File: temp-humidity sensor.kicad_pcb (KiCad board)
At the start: 2 copper layers, 36 parts, among them J1 Conn_01x02, J2 USB_C_Receptacle_USB2.0_16P, SW1 SW_Push, SW2 SW_Push, SW3 SS-12D01-G040, U1 SHT4x, U2 ESP32-C6-WROOM-1, U3 BQ24074RGT, U4 USBLC6-2SC6, U5 TPS63031DSK

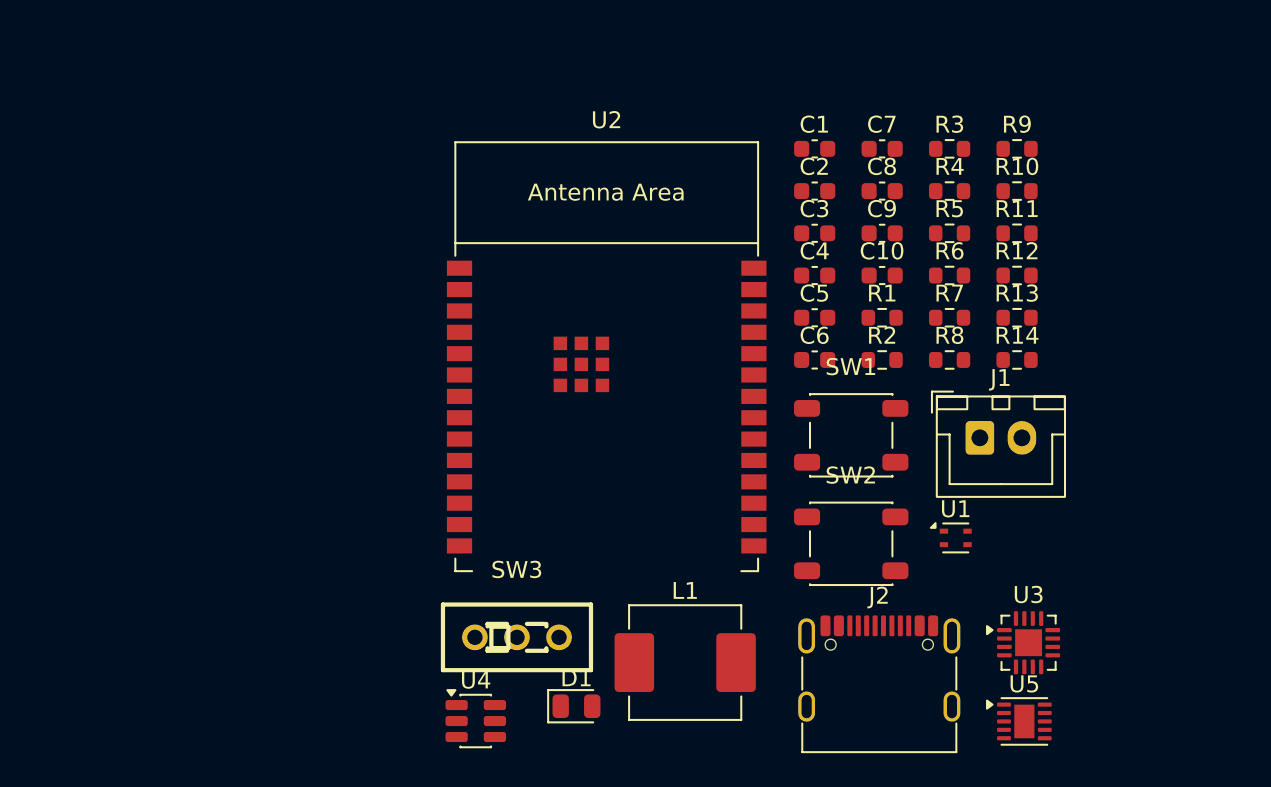
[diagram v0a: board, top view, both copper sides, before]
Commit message: Working On PCB
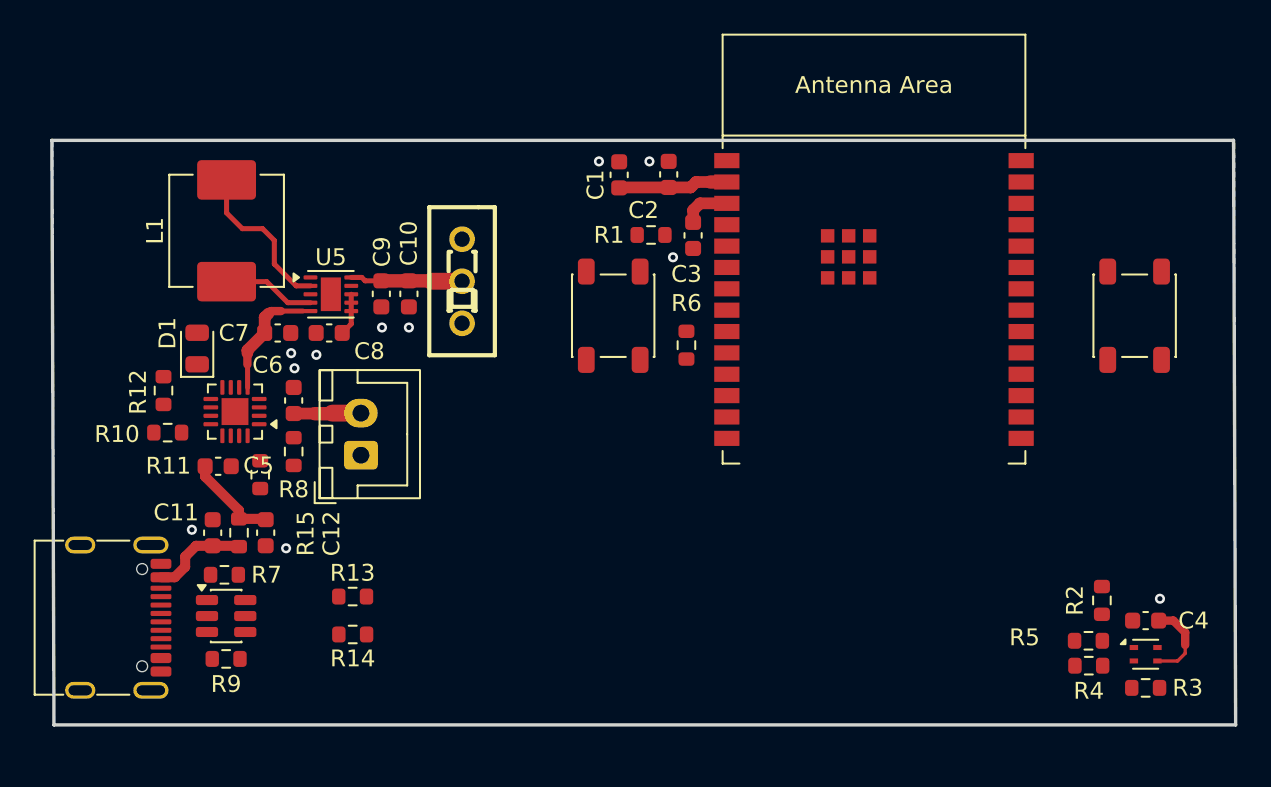
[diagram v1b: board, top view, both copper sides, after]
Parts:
- added C11: 470n, Capacitor_SMD:C_0603_1608Metric, F.Cu at (105.4, 94.6)
- added C12: 470n, Capacitor_SMD:C_0603_1608Metric, F.Cu at (108.6, 94.6)
- added R15: 0R, Resistor_SMD:R_0603_1608Metric, F.Cu at (107.0, 94.6)
- C10: value 10u -> 100n
- moved R9 56.0 mm to (106.2, 102.1), turned to 180 degrees
- moved R10 52.5 mm to (102.8, 88.6)
- moved R12 51.2 mm to (102.5, 86.1), turned to -90 degrees
- moved U3 49.1 mm to (106.8, 87.4), turned to 180 degrees
- moved U5 48.4 mm to (112.5, 80.4)
- moved R11 47.2 mm to (108.3, 91.1), turned to 90 degrees
- moved J2 46.6 mm to (98.6, 99.6), turned to -90 degrees
- moved R7 45.7 mm to (106.1, 97.1), turned to 180 degrees
- moved R13 42.8 mm to (113.8, 98.4), turned to 180 degrees
- moved R14 42.7 mm to (113.8, 100.6), turned to 180 degrees
- moved R8 39.4 mm to (110.2, 89.8), turned to -90 degrees
- moved C7 37.6 mm to (109.3, 82.7)
- moved L1 37.4 mm to (106.3, 76.6), turned to 90 degrees
- moved J1 36.8 mm to (114.2, 90.0), turned to 90 degrees
- moved C5 36.5 mm to (105.8, 90.6)
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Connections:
- C5 pad 1: /VBUS -> /VBUSF
- J1 pad 1: /BAT- -> Earth
- U2 pad 15: unconnected-(U2-GPIO9-Pad15) -> /GPIO9
- U3 pad 13: /VBUS -> /VBUSF
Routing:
- net +3V3: track 0.00 -> 11.5 mm
- net Net-(U5-L2): track 0.00 -> 9.57 mm
- net +5V: track 0.00 -> 7.45 mm
- net /VOUT: track 0.00 -> 6.65 mm
- net /VBUS: track 0.00 -> 5.79 mm
- net /VBUSF: track 0.00 -> 5.57 mm
- net Net-(U5-L1): track 0.00 -> 5.51 mm
- net /BAT+: track 0.00 -> 4.02 mm
- net /CHIP_PU: track 0.00 -> 2.89 mm
- net Net-(U5-EN): track 0.00 -> 2.52 mm
- net Earth: vias 0 -> 11
- added copper zone on B.Cu, net Earth
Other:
- board outline added: 70.4 x 34.8 mm
